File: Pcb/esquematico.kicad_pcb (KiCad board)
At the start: 2 copper layers, 117 x 63 mm, 25 parts, among them J1 Jack-DC, J2 Pin_Header, J3 Conn_01x02, J4 USB_B, J5 Conn_01x03, J6 Pin_Header, J7 Conn_01x04, SW1 SW_Push, U1 L7805, U2 AZ1117-3.3, U3 PIC18F4550-IP, Y1 Crystal 20MHz

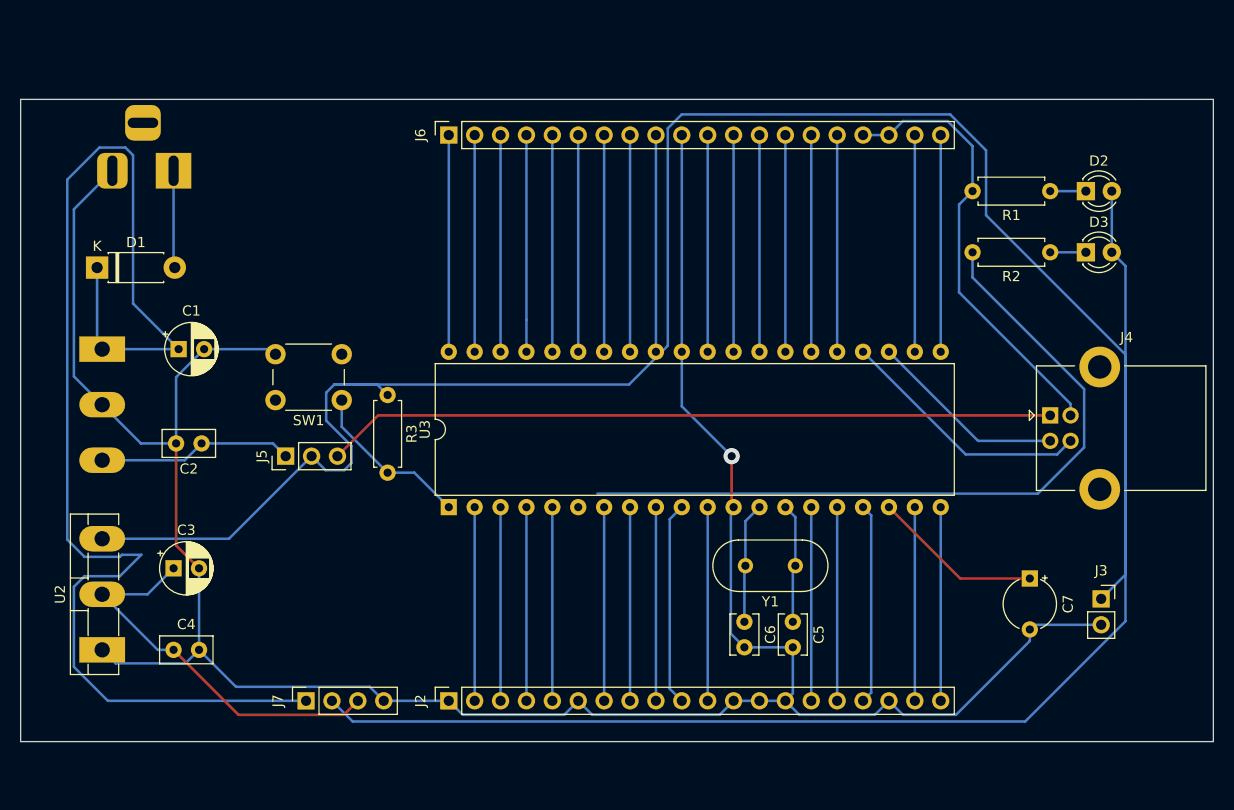
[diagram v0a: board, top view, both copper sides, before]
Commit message: ultimas correcciones
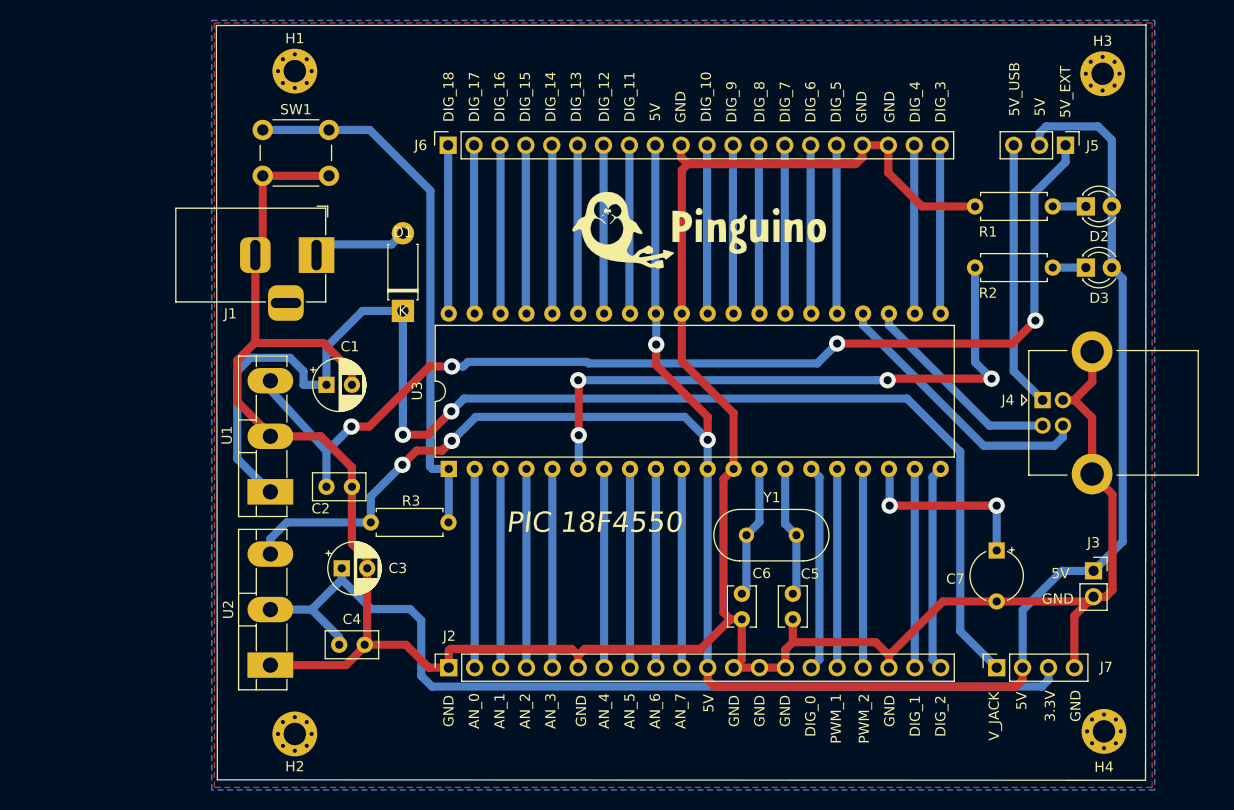
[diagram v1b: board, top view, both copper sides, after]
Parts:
- added G***: LOGO, logoPCB:logo_v3_mod, F.Cu at (113.5, 63.8)
- added G***: LOGO, logoPCB:logo_placa, F.Cu at (97.8, 94.2)
- added G***: LOGO, logoPCB:logo_placa, F.Cu at (97.0, 94.8)
- added H1: MountingHole, MountingHole:MountingHole_2.2mm_M2_Pad_Via, F.Cu at (72.9, 46.2)
- added H2: MountingHole, MountingHole:MountingHole_2.2mm_M2_Pad_Via, F.Cu at (72.9, 111.3)
- added H3: MountingHole, MountingHole:MountingHole_2.2mm_M2_Pad_Via, F.Cu at (152.1, 46.5)
- added H4: MountingHole, MountingHole:MountingHole_2.2mm_M2_Pad_Via, F.Cu at (152.3, 111.0)
- J1, U1: moved to F.Cu
- moved J5 82.4 mm to (148.5, 53.5), turned to 270 degrees
- moved J7 67.8 mm to (141.8, 104.8)
- moved D1 30.3 mm to (83.5, 69.8), turned to 90 degrees
- moved SW1 27.6 mm to (69.8, 52.0), turned to 0 degrees
- moved U1 21.6 mm to (70.5, 87.5), turned to 90 degrees
- moved U2 16.6 mm to (70.5, 104.5)
- moved C3 16.5 mm to (77.5, 95.0)
- moved J1 16.3 mm to (75.0, 64.3)
- moved C4 16.3 mm to (77.2, 102.5)
- moved C1 14.9 mm to (76.0, 77.0)
- moved C2 13.0 mm to (76.0, 87.0), turned to 0 degrees
- moved R3 12.6 mm to (80.3, 90.5), turned to 0 degrees
- moved C7 4.26 mm to (141.8, 93.2)
- moved U3 3.75 mm to (88.0, 85.2)
- moved J2 3.25 mm to (88.0, 104.8)
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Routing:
- net /+5V: track 348.7 -> 207.8 mm, vias 0 -> 4
- net /+5V_EXT: track 19.2 -> 107.2 mm, vias 0 -> 4
- net /+3.3V: track 38.6 -> 92.2 mm
- net /+5V_USB: track 71.6 -> 26.2 mm
- net /RESET: track 16.4 -> 53.6 mm
- net /LED_RUN: track 73.3 -> 61.0 mm, vias 0 -> 4
- net GND: track 289.9 -> 297.0 mm, vias 1 -> 0
- net /PIN8: track 21.3 -> 16.5 mm
- net /PIN1: track 21.3 -> 16.5 mm
- net /PIN9: track 21.3 -> 16.5 mm
- net /PIN7: track 21.3 -> 16.5 mm
- net /PIN4: track 21.3 -> 16.5 mm
- net /PIN28: track 21.3 -> 16.5 mm
- net /PIN26: track 21.3 -> 16.5 mm
- net /PIN25: track 21.3 -> 16.5 mm
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- added copper zone on B.Cu, net /+5V
- added copper zone on F.Cu, net GND
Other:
- board size 117 x 63 mm -> 91.2 x 74.1 mm
- net class Default: clearance 0.4 -> 0.6
- rule trace_clearance: 0.4 -> 0.6
- rule via_min_size: 0.4 -> 0.6
- board text added: "3.3V"
- board text added: "5V"
- board text added: "5V_EXT"
- board text added: "5V_USB"
- board text added: "AN_0"
- board text added: "AN_1"
- board text added: "AN_2"
- board text added: "AN_3"
- board text added: "AN_4"
- board text added: "AN_5"
- board text added: "AN_6"
- board text added: "AN_7"
- board text added: "DIG_0"
- board text added: "DIG_1"
- board text added: "DIG_10"
- board text added: "DIG_11"
- board text added: "DIG_12"
- board text added: "DIG_13"
- board text added: "DIG_14"
- board text added: "DIG_15"
- board text added: "DIG_16"
- board text added: "DIG_17"
- board text added: "DIG_18"
- board text added: "DIG_2"
- board text added: "DIG_3"
- board text added: "DIG_4"
- board text added: "DIG_5"
- board text added: "DIG_6"
- board text added: "DIG_7"
- board text added: "DIG_8"
- board text added: "DIG_9"
- board text added: "GND"
- board text added: "PIC 18F4550"
- board text added: "PWM_1"
- board text added: "PWM_2"
- board text added: "Replica-pinguino-pic-18f4550 NOV-2020 Diseñado-en-Argentina"
- board text added: "V_JACK"

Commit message: se agrego comentarios del diseno
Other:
- board text added: "El diseño posee los siguientes parametros: - Clearance de 0.6 mm - Ancho de pistas 0.8 mm - Grilla de 1 mm, 0.5 mm para posicionamiento y 0,5 mm para ruteo - Pad minimo 0.4 mm - PCB doble faz con componentes en una sola capa - El margen mínimo es de 0.6 mm con el borde - Fabricación manual - Sigue estandares mínimos de Ernesto Mayer S.A"
